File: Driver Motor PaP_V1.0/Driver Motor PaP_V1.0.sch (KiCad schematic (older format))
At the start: 27 parts, among them J1 Conn_01x02, J2 Conn_01x02, J3 Conn_01x02, J4 Conn_01x04, J5 Conn_01x01, J6 Conn_01x02, J7 Conn_01x02, U1 LM358, U2 LM358, U3 LM358

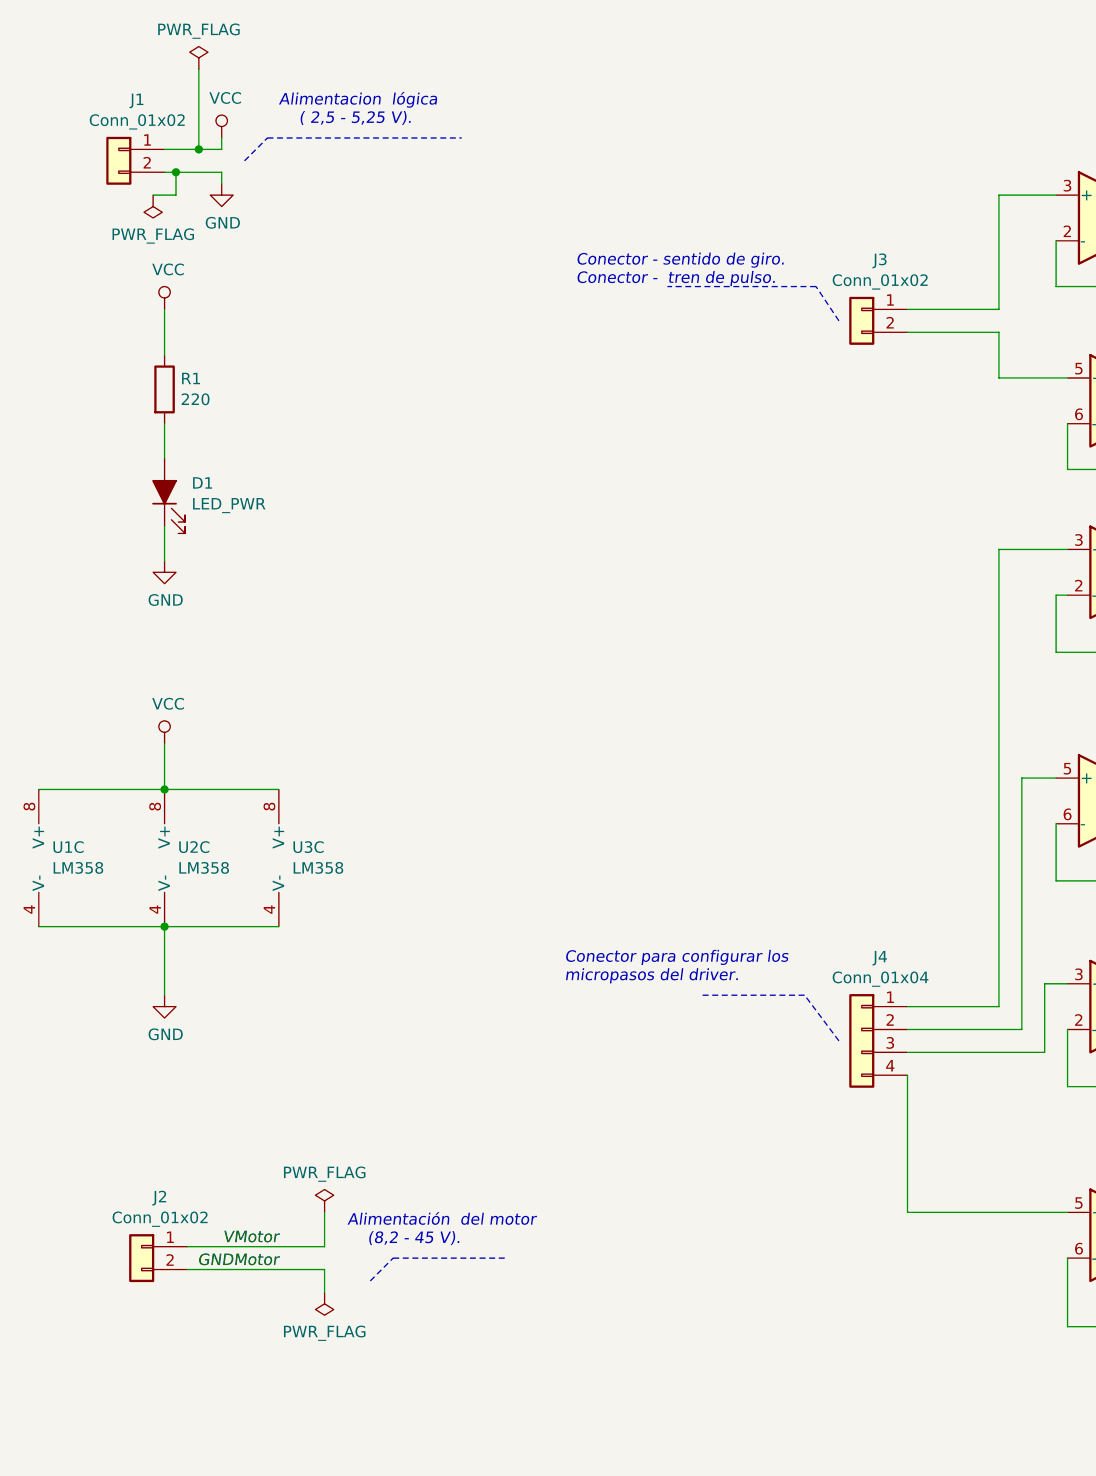
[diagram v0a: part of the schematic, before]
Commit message: Corrección que sugirio el revisador
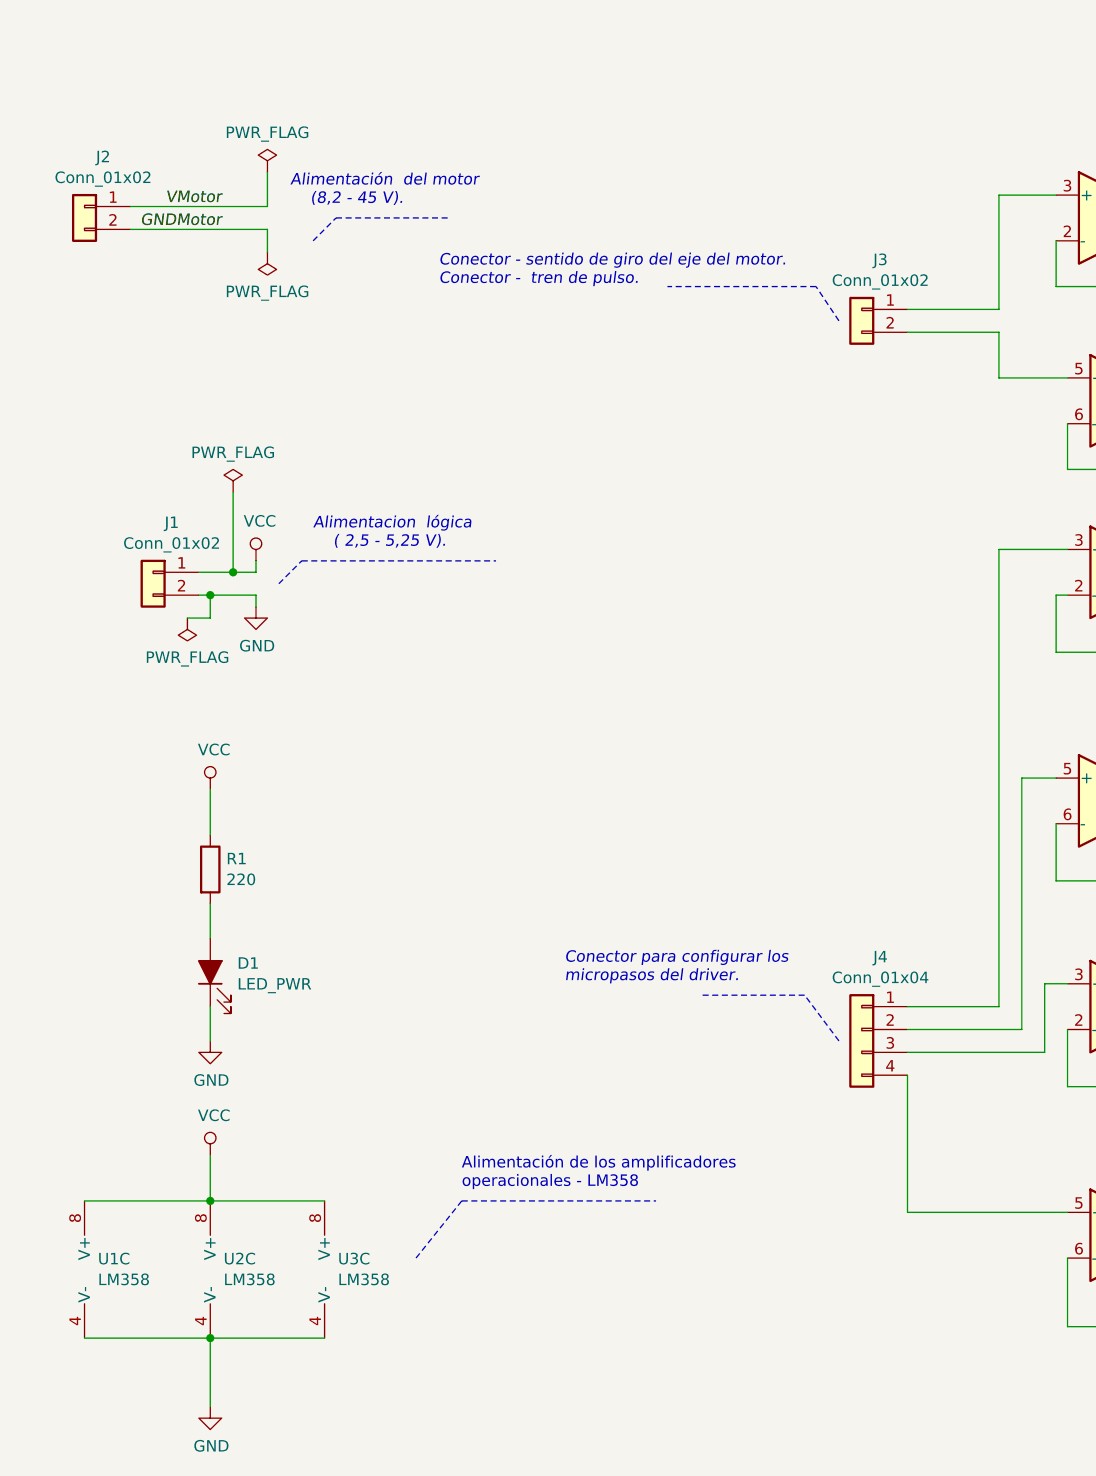
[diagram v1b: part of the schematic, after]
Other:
- note added: "Alimentación de los amplificadores \noperacionales - LM358"
- note added: "Conector - sentido de giro del eje del motor.\nConector - tren de pulso."
- note removed: "Conector - sentido de giro.\nConector - tren de pulso."
- moved on the sheet: D1, J1, J2, R1, U1C, U2C, U3C
